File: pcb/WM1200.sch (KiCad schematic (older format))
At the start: 0 parts

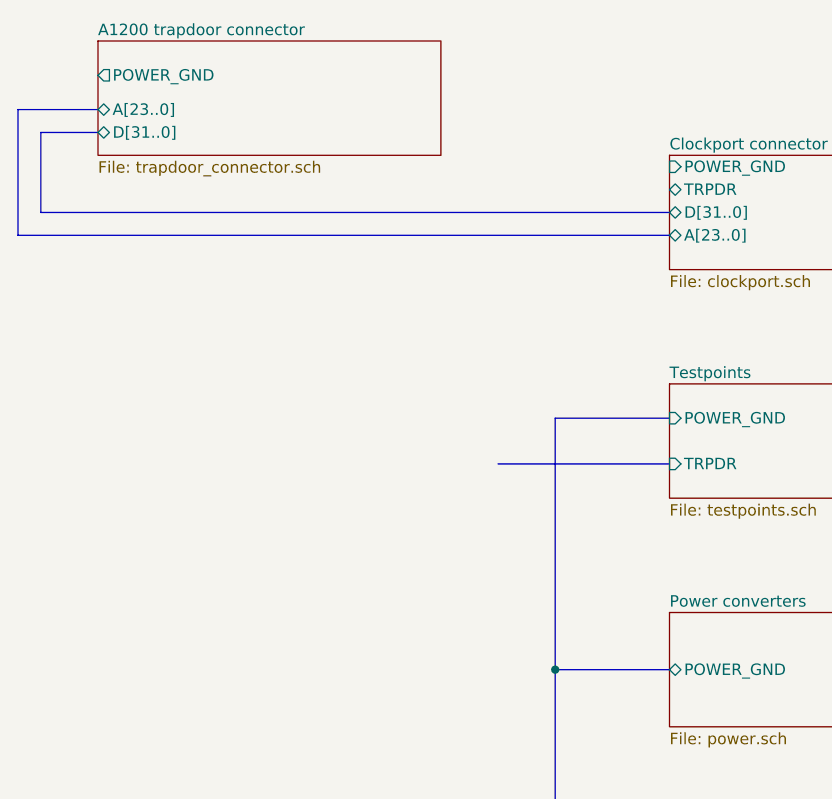
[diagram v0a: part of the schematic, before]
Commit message: wip commit (sync work between pc's)
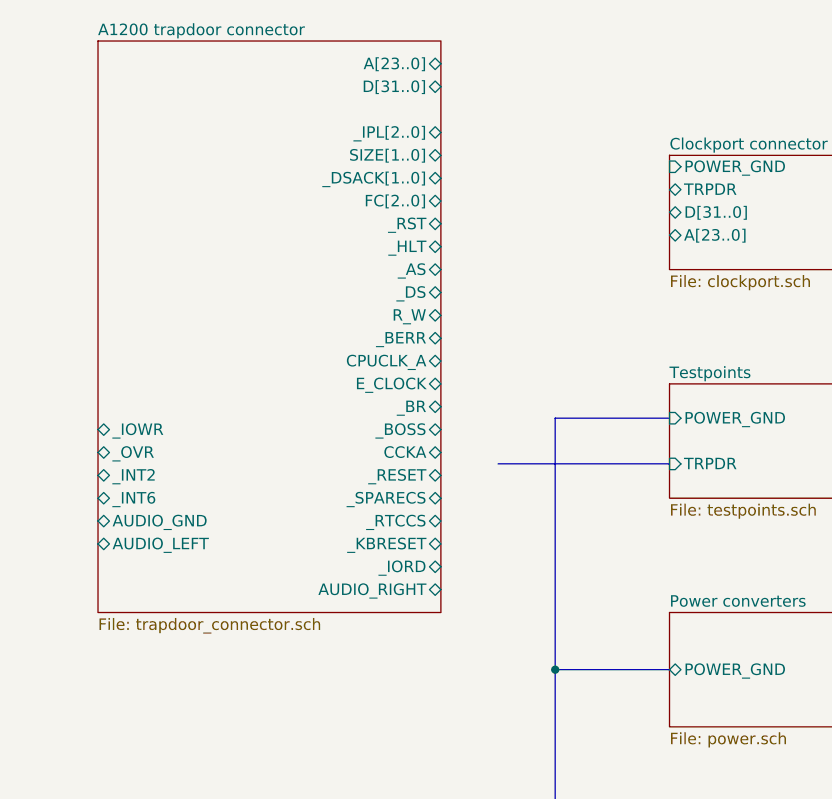
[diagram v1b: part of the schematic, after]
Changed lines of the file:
@@
 $EndDescr
-$Sheet
-S 1000 1000 1500 500
-U 5E6286C8
-F0 "A1200 trapdoor connector" 50
-F1 "trapdoor_connector.sch" 50
-F2 "POWER_GND" O L 1000 1150 50
-F3 "A[23..0]" B L 1000 1300 50
-F4 "D[31..0]" B L 1000 1400 50
-$EndSheet
 $Sheet
 S 3500 2500 1500 500
@@
 F5 "A[23..0]" B L 3500 1850 50
 $EndSheet
-Wire Bus Line
-	1000 1300 650  1300
-Wire Bus Line
-	650  1300 650  1850
-Wire Bus Line
-	650  1850 3500 1850
-Wire Bus Line
-	1000 1400 750  1400
-Wire Bus Line
-	750  1400 750  1750
-Wire Bus Line
-	750  1750 3500 1750
+$Sheet
+S 1000 1000 1500 2500
+U 5E6286C8
+F0 "A1200 trapdoor connector" 50
+F1 "trapdoor_connector.sch" 50
+F2 "A[23..0]" B R 2500 1100 50
+F3 "D[31..0]" B R 2500 1200 50
+F4 "_IPL[2..0]" B R 2500 1400 50
+F5 "SIZE[1..0]" B R 2500 1500 50
+F6 "_DSACK[1..0]" B R 2500 1600 50
+F7 "FC[2..0]" B R 2500 1700 50
+F8 "_RST" B R 2500 1800 50
+F9 "_HLT" B R 2500 1900 50
+F10 "_AS" B R 2500 2000 50
+F11 "_DS" B R 2500 2100 50
+F12 "R_W" B R 2500 2200 50
+F13 "_BERR" B R 2500 2300 50
+F14 "CPUCLK_A" B R 2500 2400 50
+F15 "E_CLOCK" B R 2500 2500 50
+F16 "_BR" B R 2500 2600 50
+F17 "_BOSS" B R 2500 2700 50
+F18 "CCKA" B R 2500 2800 50
+F19 "_RESET" B R 2500 2900 50
+F20 "_SPARECS" B R 2500 3000 50
+F21 "_RTCCS" B R 2500 3100 50
+F22 "_KBRESET" B R 2500 3200 50
+F23 "_IORD" B R 2500 3300 50
+F24 "AUDIO_RIGHT" B R 2500 3400 50
+F25 "AUDIO_LEFT" B L 1000 3200 50
+F26 "AUDIO_GND" B L 1000 3100 50
+F27 "_INT6" B L 1000 3000 50
+F28 "_INT2" B L 1000 2900 50
+F29 "_OVR" B L 1000 2800 50
+F30 "_IOWR" B L 1000 2700 50
+$EndSheet
 $EndSCHEMATC
